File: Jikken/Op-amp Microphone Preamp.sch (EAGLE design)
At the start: 29 parts, among them IC1 AD822N

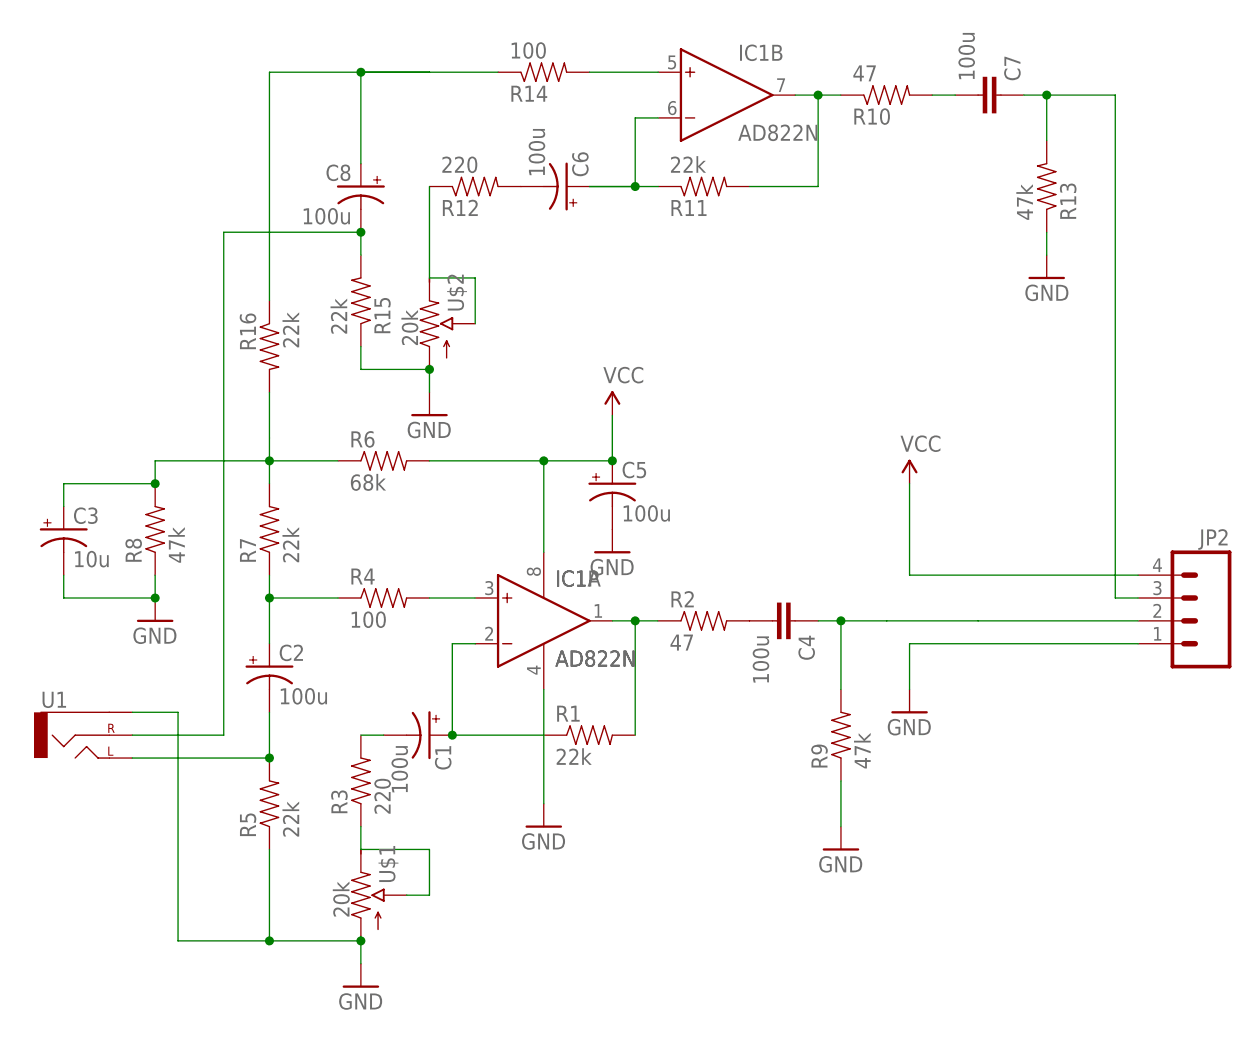
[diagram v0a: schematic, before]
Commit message: Amplifiers
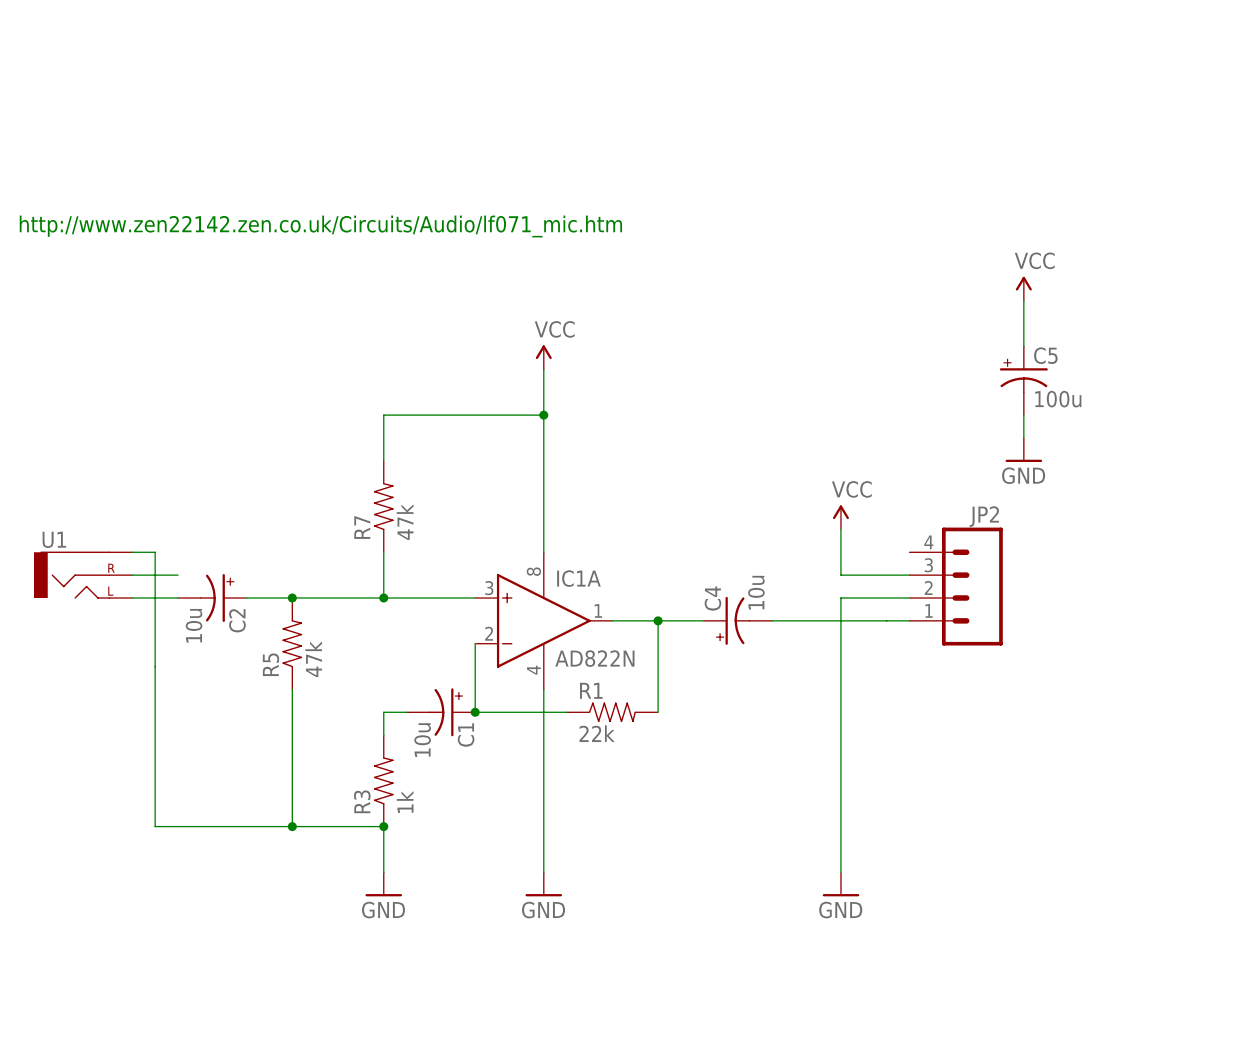
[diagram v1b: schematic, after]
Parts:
- removed C3: 10u, SparkFun:CAP_POLPTH1
- removed C6, C8: 100u, SparkFun:CAP_POLPTH1
- removed C7: 100u, capacitor-wima:C2.5/4
- removed R10, R2: 47, My Library:RESISTORPTH-1/6W
- removed R11, R15: 22k, My Library:RESISTORPTH-1/6W
- removed R12: 220, My Library:RESISTORPTH-1/6W
- removed R13, R8, R9: 47k, My Library:RESISTORPTH-1/6W
- removed R14, R4: 100, My Library:RESISTORPTH-1/6W
- removed R16: 22k, My Library:RESISTORAXIAL-0.3
- removed R6: 68k, My Library:RESISTORPTH-1/6W
- removed U$1, U$2: 20k, My Library:POT-RV16AF-20
- C1, C2: value 100u -> 10u
- C4: value 100u -> 10u; device capacitor-wima:C2.5/4 -> SparkFun:CAP_POLPTH1
- R3: value 220 -> 1k; device My Library:RESISTORPTH-1/6W -> SparkFun:RESISTORPTH-1/4W
- R5: value 22k -> 47k; device My Library:RESISTORPTH-1/6W -> SparkFun:RESISTORPTH-1/4W
- R7: value 22k -> 47k; device My Library:RESISTORAXIAL-0.3 -> SparkFun:RESISTORPTH-1/4W
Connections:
- removed net N$1: R3.1, U$1.E, U$1.S
- removed net N$10: R12.1, U$2.E, U$2.S
- removed net N$11: C6.-, R12.2
- removed net N$12: C6.+, IC1B.IN-, R11.1
- removed net N$14: IC1B.OUT, R10.1, R11.2
- removed net N$15: C8.-, R15.2, U1.RIGHT
- removed net N$16: C7.2, R10.2
- removed net N$17: C7.1, JP2.3, R13.2
- removed net N$18: C8.+, R14.1, R16.1
- removed net N$19: IC1B.IN+, R14.2
- removed net N$4: C4.2, R2.2
- removed net N$7: C2.+, R4.1, R7.1
- net GND: now also JP2.2, R3.1; no longer C3.-, JP2.1, R13.1, R15.1, R8.1, R9.1, U$1.A, U$2.A
- net N$13: now also C4.-, JP2.1; no longer C4.1, JP2.2, R9.2
- net N$3: now also C4.+; no longer R2.1
- net N$6: now also C2.+, IC1A.IN+, R7.1; no longer C2.-, U1.LEFT
- net N$8: now also C2.-, U1.LEFT; no longer IC1A.IN+, R4.2
- net N$9: now also U1.RIGHT; no longer C3.+, R16.2, R6.1, R7.2, R8.2
- net VCC: now also JP2.3, R7.2; no longer JP2.4, R6.2
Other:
- note added: "http://www.zen22142.zen.co.uk/Circuits/Audio/lf071_mic.htm"
- moved on the sheet: C1, C2, C5, JP2, R1, R3, R5, R7, U1
